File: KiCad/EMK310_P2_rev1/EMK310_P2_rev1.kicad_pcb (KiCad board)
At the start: 2 copper layers, 80 x 100 mm, 44 parts, among them J1 Conn_01x20_Socket, J2 Conn_01x02_Socket, J3 Conn_01x02_Socket, J4 Conn_01x20_Socket, J5 Conn_01x05_Socket, J6 Conn_01x04_Socket, J7 Conn_01x02_Socket, U1 PIC18F45K22, U2 Opamp_Quad, U3 Opamp_Dual

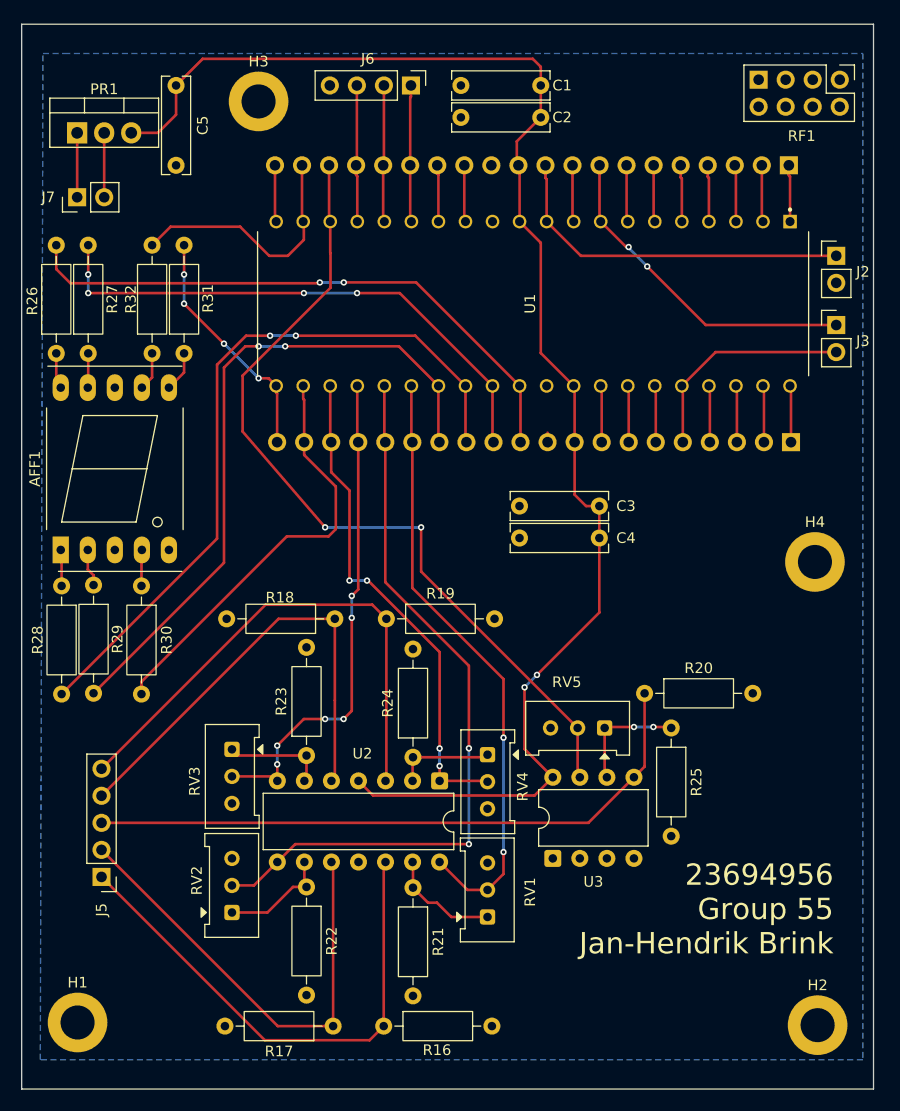
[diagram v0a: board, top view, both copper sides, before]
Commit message: work
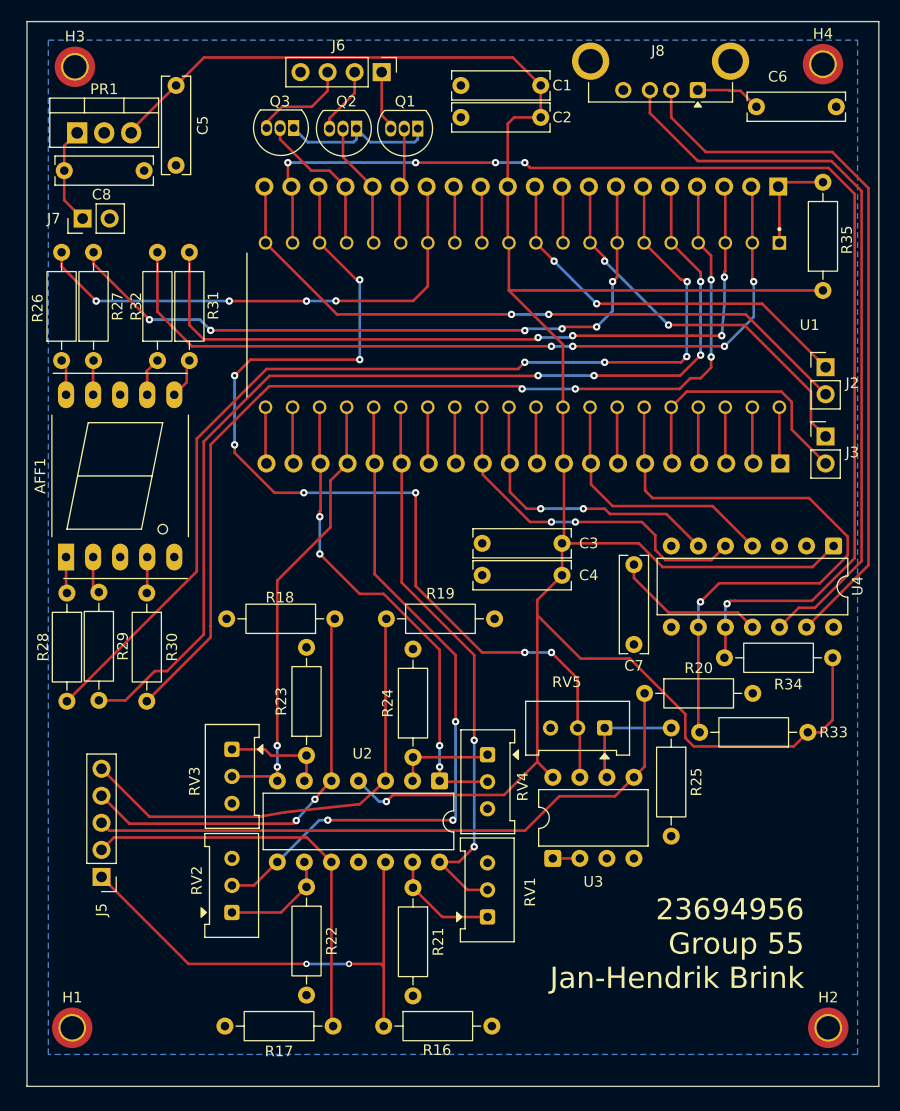
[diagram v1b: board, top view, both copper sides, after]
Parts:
- removed RF1: ESP-01-Wifi, Jan-Hendrik:PinHeader_2x04_P2.54mm_Vertical_Antenna
- added C6: 0.22uF, Capacitor_THT:C_Rect_L9.0mm_W2.5mm_P7.50mm_MKT, F.Cu at (165.0, 48.8)
- added C7: 0.22uF, Capacitor_THT:C_Rect_L9.0mm_W2.5mm_P7.50mm_MKT, F.Cu at (153.5, 91.8)
- added C8: 0.22uF, Capacitor_THT:C_Rect_L9.0mm_W2.5mm_P7.50mm_MKT, F.Cu at (107.5, 54.8)
- added J8: USB_A, Connector_USB:USB_A_Connfly_DS1095, F.Cu at (159.5, 47.2)
- added Q1: VP0610L, Package_TO_SOT_THT:TO-92L_Inline, F.Cu at (133.2, 50.8)
- added Q2: VP0610L, Package_TO_SOT_THT:TO-92L_Inline, F.Cu at (127.5, 50.8)
- added Q3: VP0610L, Package_TO_SOT_THT:TO-92L_Inline, F.Cu at (121.5, 50.8)
- added R33: 10k, Resistor_THT:R_Axial_DIN0207_L6.3mm_D2.5mm_P10.16mm_Horizontal, F.Cu at (169.8, 107.5)
- added R34: 10k, Resistor_THT:R_Axial_DIN0207_L6.3mm_D2.5mm_P10.16mm_Horizontal, F.Cu at (172.2, 100.5)
- added R35: 10k, Resistor_THT:R_Axial_DIN0207_L6.3mm_D2.5mm_P10.16mm_Horizontal, F.Cu at (171.2, 66.0)
- added U4: MCP2221AxP, Package_DIP:DIP-14_W7.62mm, F.Cu at (172.2, 90.0)
- C5: value C_Small -> 10uF
- H1, H2, H3, H4: footprint MountingHole:MountingHole_3.2mm_M3_DIN965_Pad -> MountingHole:MountingHole_2.2mm_M2_DIN965_Pad_TopOnly
- moved H4 46.8 mm to (171.2, 44.8)
- moved H3 17.6 mm to (101.0, 45.0)
- moved J2 10.5 mm to (171.5, 73.2)
- moved J3 10.5 mm to (171.5, 79.7)
- moved C3 4.95 mm to (146.8, 89.8)
- moved C4 4.95 mm to (146.8, 92.8)
- moved J6 3.02 mm to (129.8, 45.5)
- moved J1 2.24 mm to (167.2, 82.2)
- moved J4 2.24 mm to (167.1, 56.2)
- moved U1 2.24 mm to (143.0, 69.2)
- moved J7 2.07 mm to (101.7, 59.2)
- moved H2 1.03 mm to (171.8, 135.2)
- moved AFF1 0.84 mm to (100.2, 91.0)
- moved R26 0.84 mm to (99.8, 72.6)
- moved R27 0.84 mm to (102.8, 72.6)
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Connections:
- net Net-(J1-Pin_6) renamed /SDA
- J4 pad 19: Net-(J4-Pin_19) -> /SCL
- J6 pad 1: /LEDR -> Net-(J6-Pin_1)
- J6 pad 2: /LEDG -> Net-(J6-Pin_2)
- J6 pad 3: /LEDB -> Net-(J6-Pin_3)
- R26 pad 2: Net-(J1-Pin_11) -> Net-(J4-Pin_14)
- R27 pad 2: Net-(J1-Pin_12) -> Net-(J4-Pin_7)
- R28 pad 2: Net-(J1-Pin_13) -> Net-(J4-Pin_6)
- R29 pad 2: Net-(J1-Pin_14) -> Net-(J4-Pin_5)
- R30 pad 2: Net-(J1-Pin_19) -> Net-(J4-Pin_4)
- R31 pad 2: Net-(J1-Pin_20) -> Net-(J4-Pin_3)
- R32 pad 2: Net-(J4-Pin_19) -> Net-(J4-Pin_2)
- U1 pad 19: Net-(J4-Pin_19) -> /SCL
- U3 pad 1: unconnected-(U3-Pad1) -> Net-(U3A--)
- U3 pad 2: unconnected-(U3A---Pad2) -> Net-(U3A--)
- U3 pad 3: unconnected-(U3A-+-Pad3) -> GNDREF
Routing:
- net /SCL: track 0.00 -> 115.3 mm, vias 0 -> 5
- net /Vdd: track 138.4 -> 246.0 mm, vias 2 -> 1
- net Net-(J4-Pin_5): track 5.33 -> 97.6 mm, vias 0 -> 4
- net Net-(J4-Pin_6): track 5.33 -> 96.9 mm, vias 0 -> 4
- net Net-(J4-Pin_4): track 5.33 -> 94.3 mm, vias 0 -> 4
- net Net-(J4-Pin_2): track 5.33 -> 76.4 mm, vias 0 -> 4
- net Net-(J8-D+): track 0.00 -> 70.1 mm
- net Net-(J8-D-): track 0.00 -> 67.5 mm
- net Net-(J4-Pin_3): track 5.33 -> 71.7 mm, vias 0 -> 4
- net Net-(J1-Pin_13): track 68.7 -> 5.32 mm, vias 2 -> 0
- net Net-(J4-Pin_7): track 5.33 -> 65.1 mm, vias 0 -> 6
- net /MOTOR_1_B: track 5.33 -> 63.8 mm, vias 0 -> 2
- net Net-(J1-Pin_14): track 63.5 -> 5.32 mm, vias 2 -> 0
- net /SDA: track 5.32 -> 58.5 mm, vias 0 -> 1
- net Net-(J4-Pin_14): track 5.33 -> 47.0 mm, vias 0 -> 4
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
